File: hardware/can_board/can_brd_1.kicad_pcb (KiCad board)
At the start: 2 copper layers, 32.1 x 10.9 mm, 13 parts, among them M471 CONN_1, P471 CONN_4, P472 CONN_2, P473 CONN_2, U471 SN65HVD230

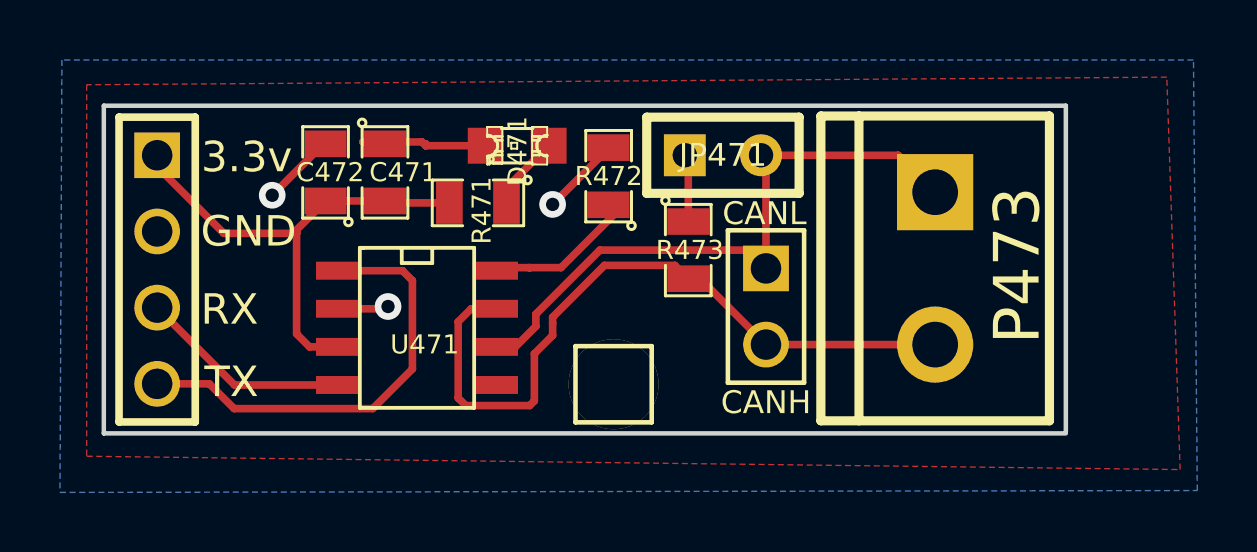
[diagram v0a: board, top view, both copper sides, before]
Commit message: update pcb files
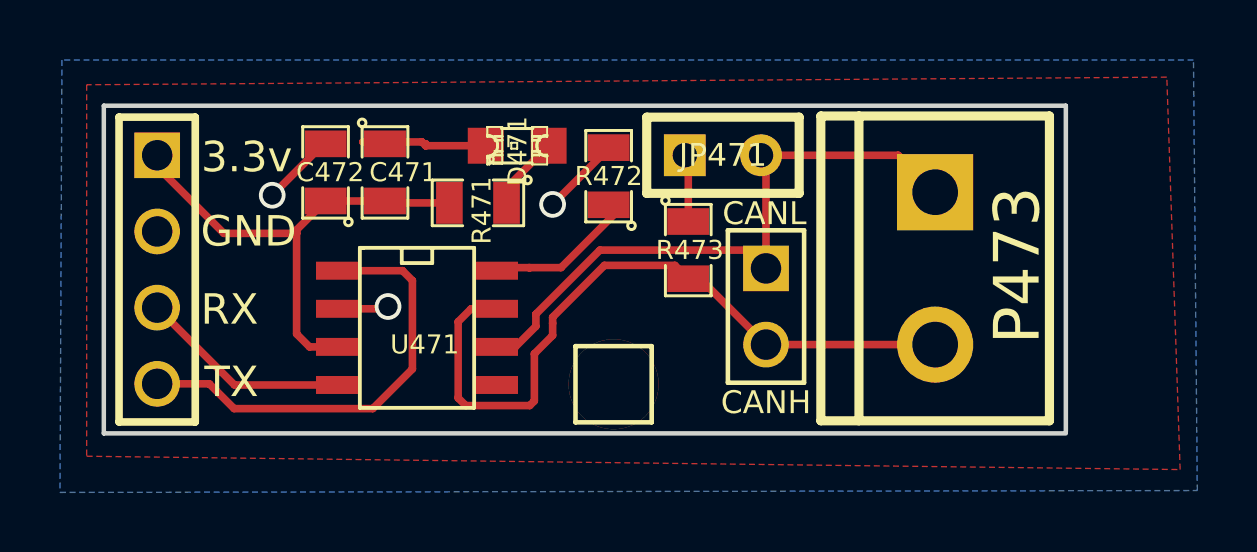
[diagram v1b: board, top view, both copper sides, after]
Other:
- net class Default removed
